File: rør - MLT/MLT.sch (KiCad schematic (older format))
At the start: 44 parts, among them J1 PJ301M-12, J10 PJ301M-12, J11 PJ301M-12, J12 PJ301M-12, J2 PJ301M-12, J3 PJ301M-12, J4 PJ301M-12, J5 PJ301M-12, J6 PJ301M-12, J7 PJ301M-12, J8 PJ301M-12, J9 PJ301M-12, U1 TL074, U2 TL074, U3 TL074

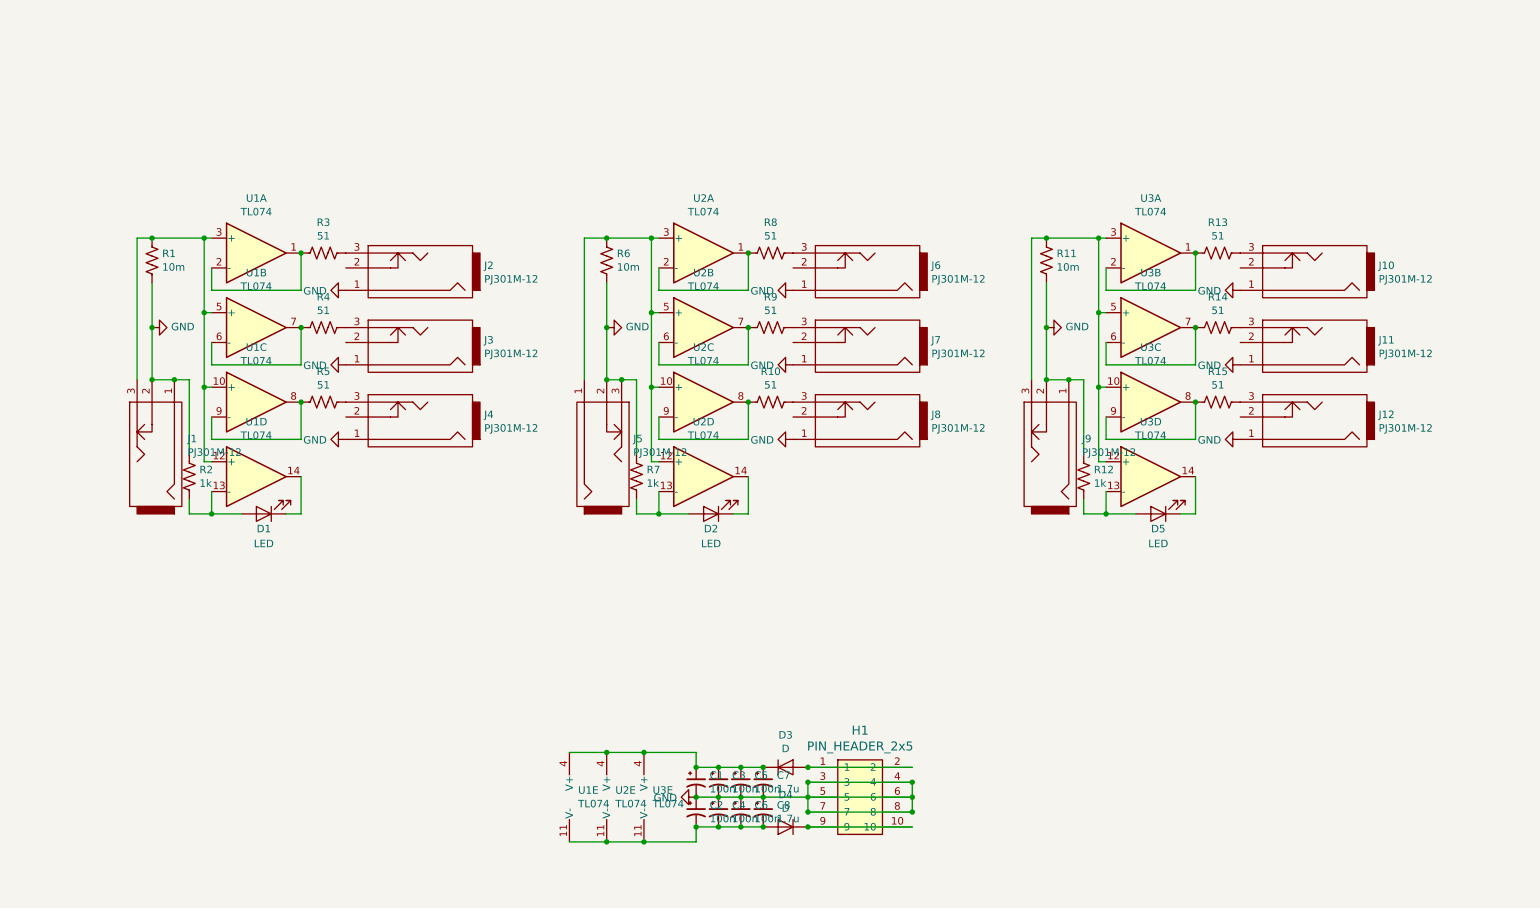
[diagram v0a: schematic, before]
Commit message: hmm
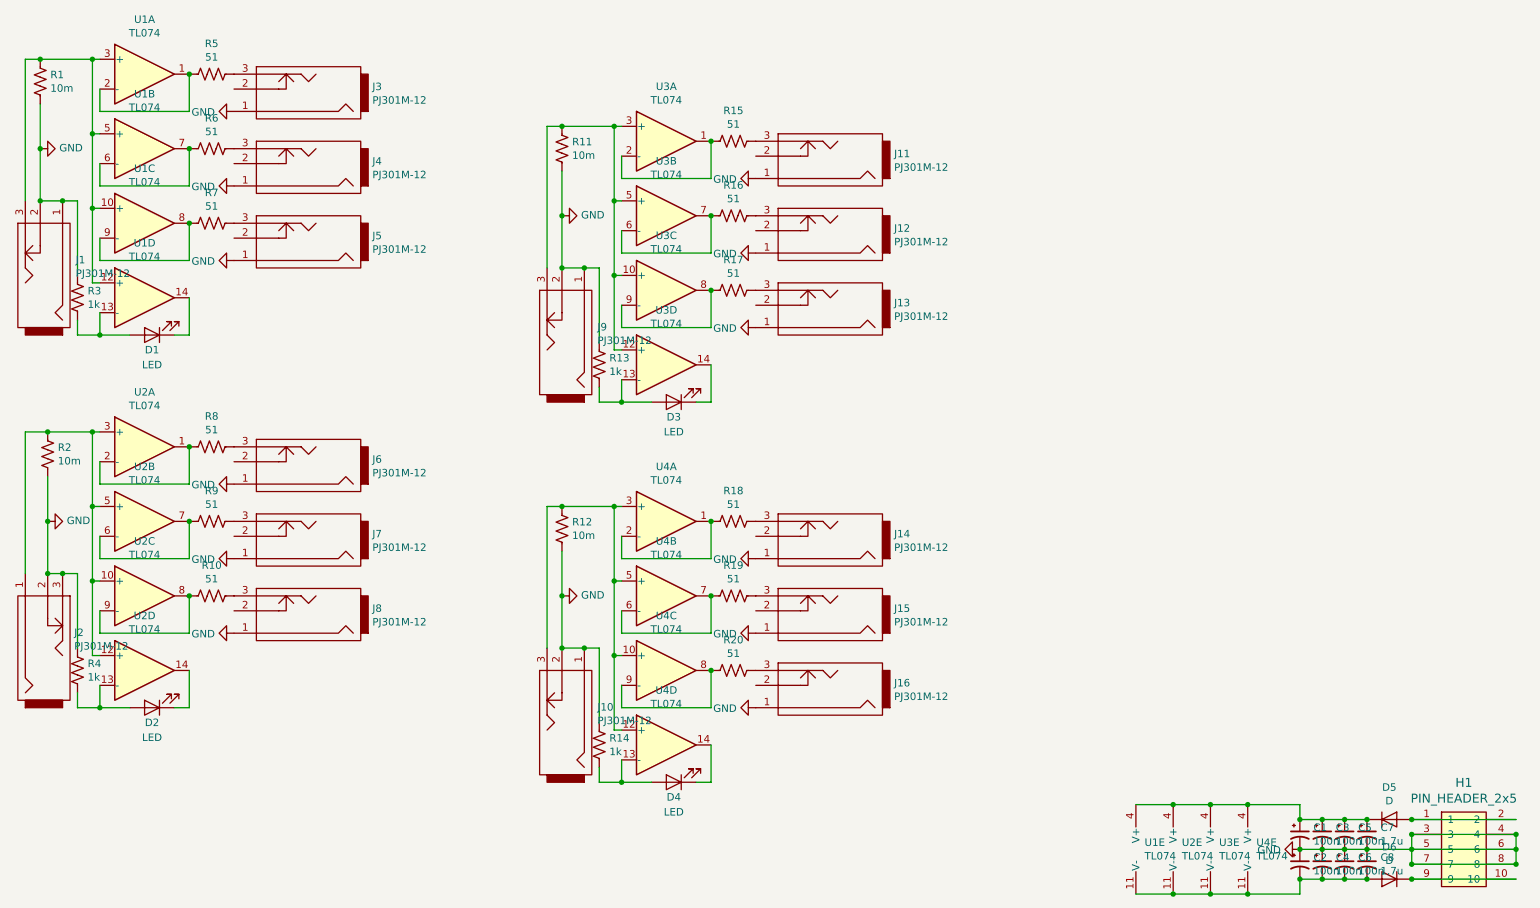
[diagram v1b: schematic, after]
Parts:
- added D4: LED, LED_THT:LED_D3.0mm_FlatTop, symbol Device:LED
- added J10, J14, J15, J16: PJ301M-12, eurorack:PJ301M-12, symbol MLT-rescue:PJ301M-12-eurocad
- added R12: 10m, Resistor_SMD:R_0603_1608Metric_Pad1.05x0.95mm_HandSolder, symbol Device:R_US
- added R14: 1k, Resistor_SMD:R_0603_1608Metric_Pad1.05x0.95mm_HandSolder, symbol Device:R_US
- added R18, R19, R20: 51, Resistor_SMD:R_0603_1608Metric_Pad1.05x0.95mm_HandSolder, symbol Device:R_US
- added unit 5 of U1
- added unit 1 of U4
- added unit 2 of U4
- added unit 3 of U4
- added unit 4 of U4
- renumbered D5 to D3, D3 to D5, D4 to D6, J10 to J11, J11 to J12, J12 to J13, J5 to J2, J2 to J3, J3 to J4, J4 to J5, R12 to R13, R13 to R15, R14 to R16, R15 to R17, R6 to R2, R2 to R3, R7 to R4, R3 to R5, R4 to R6, R5 to R7, U1 to U2, U2 to U3, U3 to U4
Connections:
- net GND: now also J10.1, J10.2, J14.1, J15.1, J16.1, R12.2, R14.1
- net at C2.2, C4.2, C6.2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: now also U1.11 (V-)
- net at C1.1, C3.1, C5.1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: now also U1.4 (V+)
- new net: R18.1, U4.1, U4.2 (-)
- new net: J10.3, R12.1, U4.10 (+), U4.12 (+), U4.3 (+), U4.5 (+)
- new net: R19.1, U4.6 (-), U4.7
- new net: R20.1, U4.8, U4.9 (-)
- new net: D4.2 (A), R14.2, U4.13 (-)
- new net: D4.1 (K), U4.14
- new net: J14.3, R18.2
- new net: J15.3, R19.2
- new net: J16.3, R20.2
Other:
- moved on the sheet: C1, C2, C3, C4, C5, C6, C7, C8, D1, D2, D3, D5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
